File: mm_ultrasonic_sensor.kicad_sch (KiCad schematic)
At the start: 3 parts, among them U4 HC-SR04

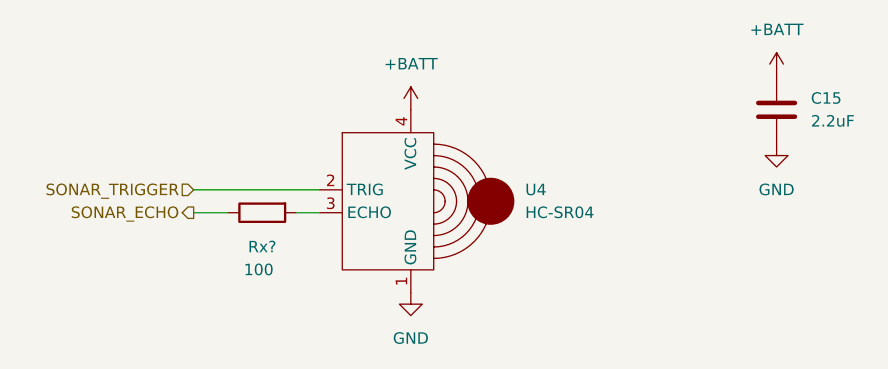
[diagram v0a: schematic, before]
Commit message: tp5
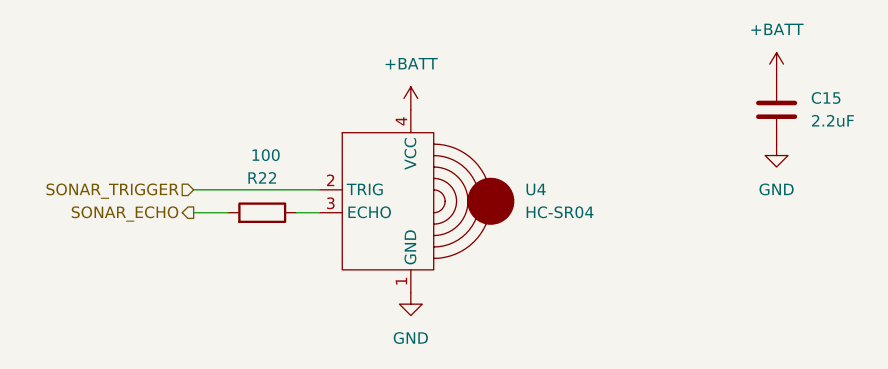
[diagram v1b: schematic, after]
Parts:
- gave numbers to parts that had none: 1
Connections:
- net SONAR_ECHO: now also R22.2; no longer R22.1
- net at U4.3 (ECHO): now also R22.1; no longer R22.2
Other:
- moved on the sheet: R22
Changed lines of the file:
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@@
     (pin "3")
     (instances
-      (project "tp2"
+      (project "tp3"
         (path "/d8fa4cba-2469-4231-847f-065b6b829f44/224298a9-7d6e-4a70-a0a5-f2614895ec28"
           (reference "U4") (unit 1)
@@
     (pin "1")
     (instances
-      (project "tp2"
+      (project "tp3"
         (path "/d8fa4cba-2469-4231-847f-065b6b829f44/224298a9-7d6e-4a70-a0a5-f2614895ec28"
           (reference "#PWR034") (unit 1)
@@
     (pin "2")
     (instances
-      (project "tp2"
+      (project "tp3"
         (path "/d8fa4cba-2469-4231-847f-065b6b829f44/224298a9-7d6e-4a70-a0a5-f2614895ec28"
           (reference "C15") (unit 1)
@@
     (pin "1")
     (instances
-      (project "tp2"
+      (project "tp3"
         (path "/d8fa4cba-2469-4231-847f-065b6b829f44/224298a9-7d6e-4a70-a0a5-f2614895ec28"
           (reference "#PWR035") (unit 1)
@@
     (pin "1")
     (instances
-      (project "tp2"
+      (project "tp3"
         (path "/d8fa4cba-2469-4231-847f-065b6b829f44/224298a9-7d6e-4a70-a0a5-f2614895ec28"
           (reference "#PWR037") (unit 1)
@@
     )
   )
-  (symbol (lib_id "Device:R") (at 116.84 91.44 90) (mirror x) (unit 1)
+  (symbol (lib_id "Device:R") (at 116.84 91.44 270) (mirror x) (unit 1)
     (in_bom yes) (on_board yes) (dnp no)
-    (property "Reference" "Rx?" (at 116.84 95.25 90)
+    (property "Reference" "R22" (at 116.84 87.63 90)
       (effects (font (size 1.27 1.27)))
     )
-    (property "Value" "100 " (at 118.11 97.79 90)
+    (property "Value" "100 " (at 115.57 85.09 90)
       (effects (font (size 1.27 1.27)) (justify left))
     )
-    (property "Footprint" "Resistor_SMD:R_0603_1608Metric" (at 116.84 89.662 90)
+    (property "Footprint" "Resistor_SMD:R_0603_1608Metric" (at 116.84 93.218 90)
       (effects (font (size 1.27 1.27)) hide)
     )
@@
     (pin "1")
     (instances
-      (project "tp2"
-        (path "/d8fa4cba-2469-4231-847f-065b6b829f44/d17bb1c7-f68a-465e-9a17-5858ef86fc30"
-          (reference "Rx?") (unit 1)
-        )
+      (project "tp3"
         (path "/d8fa4cba-2469-4231-847f-065b6b829f44/224298a9-7d6e-4a70-a0a5-f2614895ec28"
           (reference "R22") (unit 1)
@@
     (pin "1")
     (instances
-      (project "tp2"
+      (project "tp3"
         (path "/d8fa4cba-2469-4231-847f-065b6b829f44/224298a9-7d6e-4a70-a0a5-f2614895ec28"
           (reference "#PWR036") (unit 1)
